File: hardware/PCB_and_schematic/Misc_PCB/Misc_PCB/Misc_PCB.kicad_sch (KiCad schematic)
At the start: 0 parts

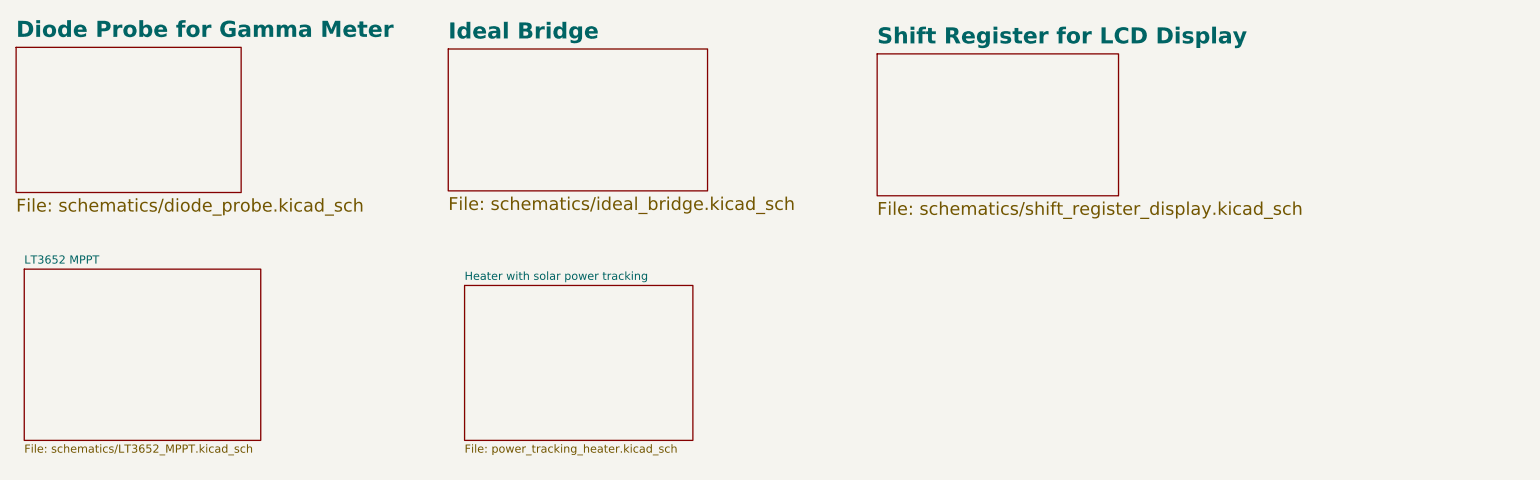
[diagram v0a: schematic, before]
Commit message: progress with esp power pcb
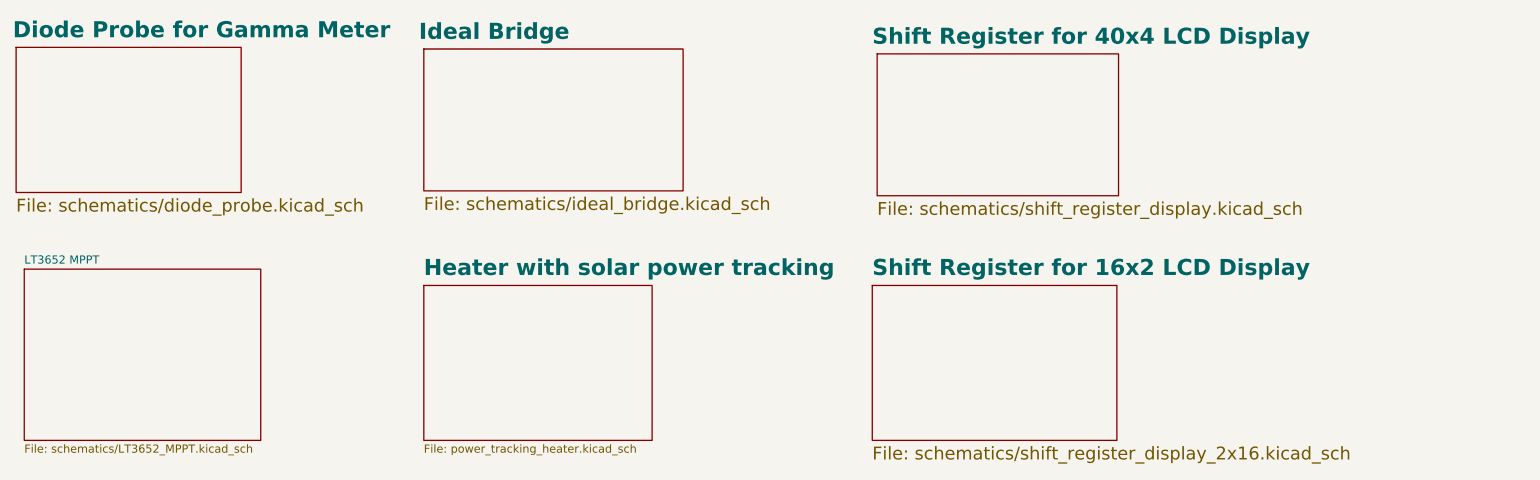
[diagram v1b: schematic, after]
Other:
- sheet Shift Register for LCD Display renamed Shift Register for 40x4 LCD Display
- added sheet Shift Register for 16x2 LCD Display (schematics/shift_register_display_2x16.kicad_sch)
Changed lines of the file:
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@@
 	(paper "A4")
 	(sheet
-		(at 88.9 63.5)
+		(at 82.55 63.5)
 		(size 35.56 24.13)
 		(fields_autoplaced yes)
@@
 		)
 		(property "Sheetname" "Heater with solar power tracking"
-			(at 88.9 62.7884 0)
-			(effects
-				(font
-					(size 1.27 1.27)
+			(at 82.55 62.1734 0)
+			(effects
+				(font
+					(size 2.5 2.5)
+					(bold yes)
 				)
 				(justify left bottom)
@@
 		)
 		(property "Sheetfile" "power_tracking_heater.kicad_sch"
-			(at 88.9 88.2146 0)
+			(at 82.55 88.2146 0)
 			(effects
 				(font
@@
 	)
 	(sheet
-		(at 86.36 26.67)
+		(at 152.4 63.5)
+		(size 38.1 24.13)
+		(fields_autoplaced yes)
+		(stroke
+			(width 0.1524)
+			(type solid)
+		)
+		(fill
+			(color 0 0 0 0.0000)
+		)
+		(property "Sheetname" "Shift Register for 16x2 LCD Display"
+			(at 152.4 62.1734 0)
+			(effects
+				(font
+					(size 2.5 2.5)
+					(bold yes)
+				)
+				(justify left bottom)
+			)
+		)
+		(property "Sheetfile" "schematics/shift_register_display_2x16.kicad_sch"
+			(at 152.4 88.5066 0)
+			(effects
+				(font
+					(size 2 2)
+				)
+				(justify left top)
+			)
+		)
+		(instances
+			(project "Misc_PCB"
+				(path "/7b59bc46-701c-4caa-9db8-f0eec290561d"
+					(page "7")
+				)
+			)
+		)
+	)
+	(sheet
+		(at 82.55 26.67)
 		(size 40.386 22.098)
-		(fields_autoplaced yes)
 		(stroke
 			(width 0.1524)
@@
 		)
 		(property "Sheetname" "Ideal Bridge"
-			(at 86.36 25.3434 0)
+			(at 81.788 25.4 0)
 			(effects
 				(font
@@
 		)
 		(property "Sheetfile" "schematics/ideal_bridge.kicad_sch"
-			(at 86.36 49.6446 0)
+			(at 82.55 49.6446 0)
 			(effects
 				(font
@@
 		(at 19.05 26.416)
 		(size 35.052 22.606)
-		(fields_autoplaced yes)
 		(stroke
 			(width 0.1524)
@@
 		)
 		(property "Sheetname" "Diode Probe for Gamma Meter"
-			(at 19.05 25.0894 0)
+			(at 18.542 25.146 0)
 			(effects
 				(font
@@
 		(at 153.162 27.432)
 		(size 37.592 22.098)
-		(fields_autoplaced yes)
-		(stroke
-			(width 0.1524)
-			(type solid)
-		)
-		(fill
-			(color 0 0 0 0.0000)
-		)
-		(property "Sheetname" "Shift Register for LCD Display"
-			(at 153.162 26.1054 0)
-			(effects
-				(font
+		(stroke
+			(width 0.1524)
+			(type solid)
+		)
+		(fill
+			(color 0 0 0 0.0000)
+		)
+		(property "Sheetname" "Shift Register for 40x4 LCD Display"
+			(at 152.4 26.162 0)
+			(effects
+				(font
